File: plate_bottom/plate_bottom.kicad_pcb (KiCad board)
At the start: 2 copper layers, 180.6 x 117.9 mm, 13 parts

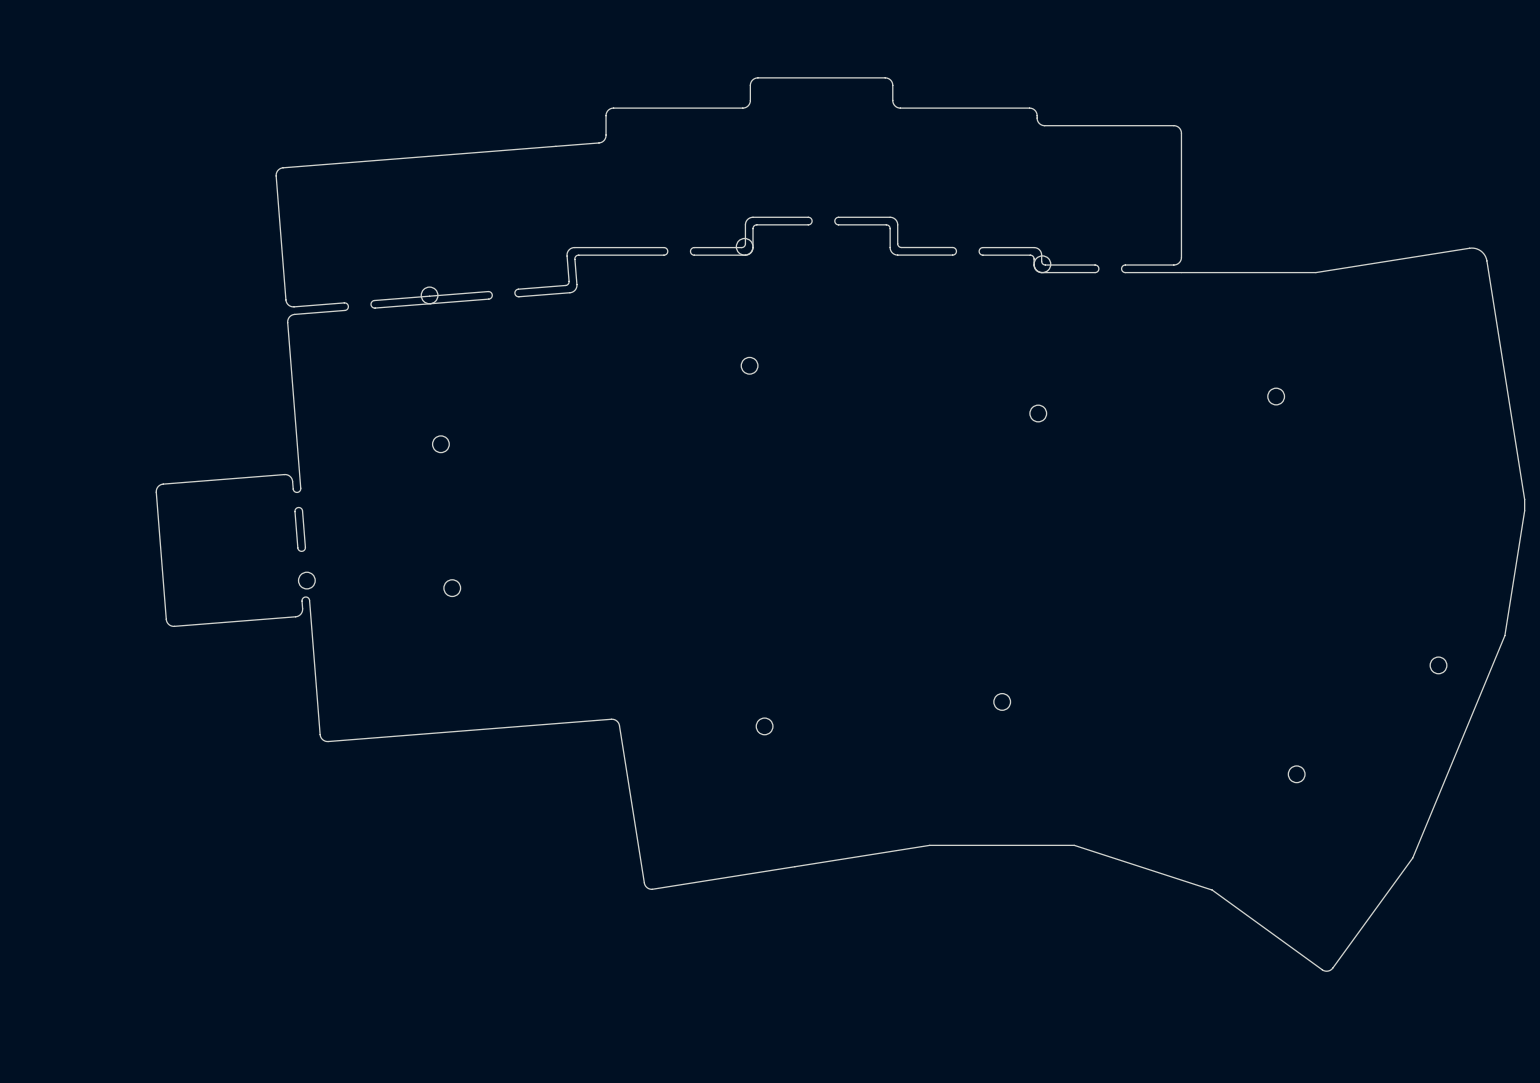
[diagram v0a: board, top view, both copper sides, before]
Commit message: Plates
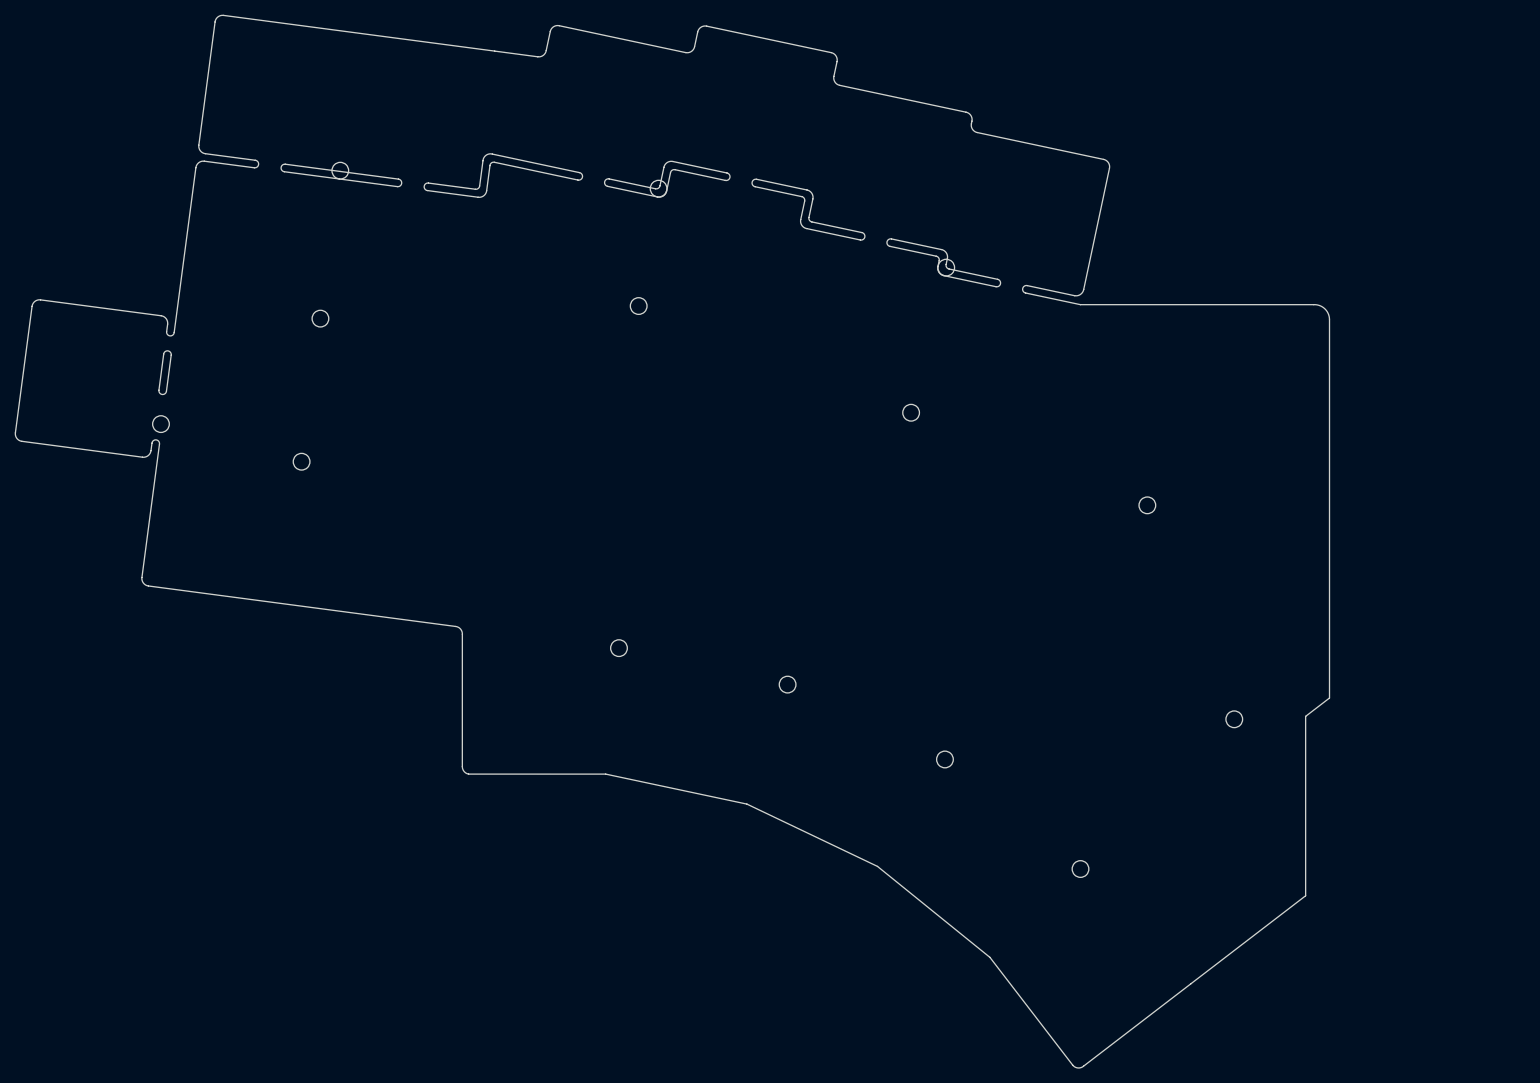
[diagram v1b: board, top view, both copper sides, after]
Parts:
- added HM14: CaseHole, used_footprints:M2_HOLE_PCB, F.Cu at (178.4, 120.5)
- moved HM3 54.4 mm to (196.3, 135.0), turned to 352.5 degrees
- moved HM4 28.4 mm to (157.7, 110.6), turned to 348 degrees
- moved HM5 28.2 mm to (75.0, 76.2), turned to 352.5 degrees
- moved HM6 26.0 mm to (93.5, 81.2), turned to 352.5 degrees
- moved HM8 23.0 mm to (96.0, 62.3), turned to 352.5 degrees
- moved H16 22.3 mm to (205.2, 87.0), turned to 348 degrees
- moved HM13 21.8 mm to (135.4, 105.8), turned to 342 degrees
- moved HM7 20.2 mm to (98.6, 42.8), turned to 352.5 degrees
- moved HM10 16.8 mm to (174.0, 74.7), turned to 348 degrees
- moved HM11 16.6 mm to (138.0, 60.7), turned to 348 degrees
- moved HM9 13.7 mm to (140.6, 45.2), turned to 348 degrees
- moved HM2 12.7 mm to (178.6, 55.6), turned to 2.5 degrees
- moved HM1 11.0 mm to (216.6, 115.2), turned to 340.5 degrees
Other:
- board size 180.6 x 117.9 mm -> 173.5 x 138.9 mm
